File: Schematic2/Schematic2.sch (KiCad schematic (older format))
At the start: 52 parts, among them SW1 Rotary_Encoder_Switch, U1 Kailhlowprofile, U10 Kailhlowprofile, U11 Kailhlowprofile, U12 Kailhlowprofile, U13 Kailhlowprofile, U14 Kailhlowprofile, U15 Kailhlowprofile, U16 Kailhlowprofile, U17 Kailhlowprofile, U18 Kailhlowprofile, U19 Kailhlowprofile, U2 Kailhlowprofile, U20 Kailhlowprofile, U3 Kailhlowprofile, U4 Kailhlowprofile, U5 Kailhlowprofile, U6 Kailhlowprofile, U7 Kailhlowprofile, U8 Kailhlowprofile, U9 Kailhlowprofile

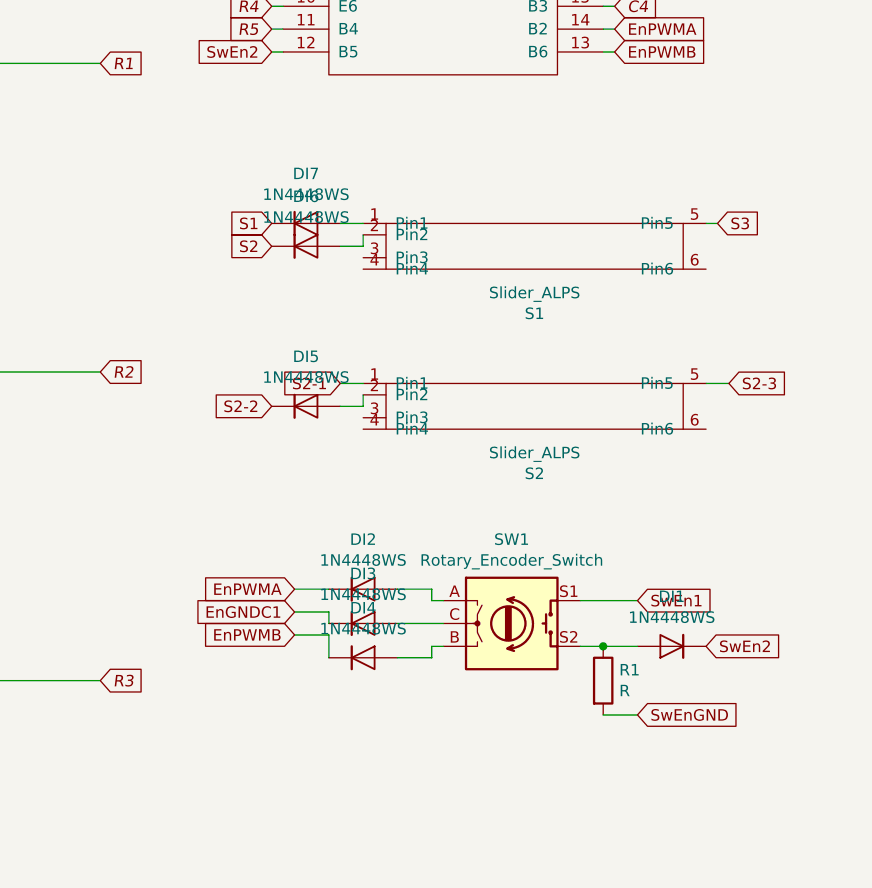
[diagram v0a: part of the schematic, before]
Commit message: The final countdown
The diamond deluxe of FINAL
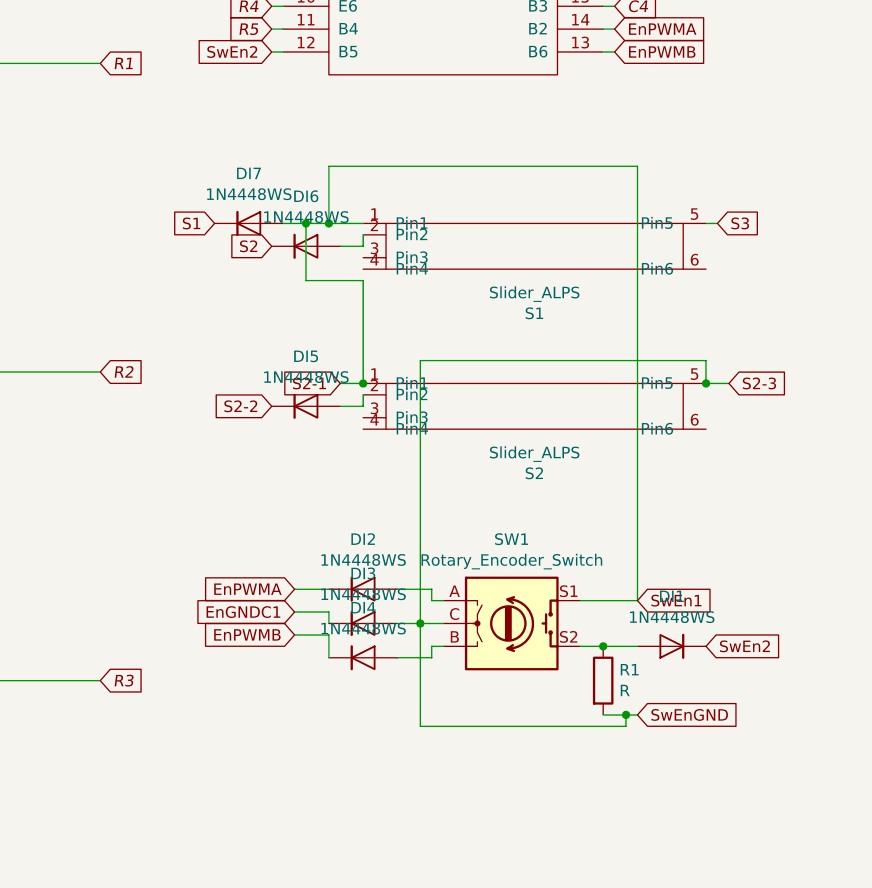
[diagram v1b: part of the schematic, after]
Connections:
- net EnGNDC1: now also DI3.2 (A), SW1.C
- net S1: now also DI7.2 (A), S1.1 (Pin1)
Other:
- moved on the sheet: DI7
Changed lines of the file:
@@
 S3
-Wire Wire Line
-	8850 2650 8950 2650
 Wire Wire Line
 	8850 2750 8950 2750
@@
 Text GLabel 8550 2750 0    50   Input ~ 0
 S2
-Text GLabel 8550 2650 0    50   Input ~ 0
+Text GLabel 8300 2650 0    50   Input ~ 0
 S1
 Text GLabel 10200 1200 2    50   Input ~ 0
@@
 	10000 4500 10150 4500
 Wire Wire Line
-	10000 4800 10150 4800
+	10000 4800 10100 4800
 Text GLabel 10800 900  2    50   Input ~ 0
 SwEnGND
@@
 Wire Wire Line
 	10000 950  10000 900
-Text GLabel 10800 700  2    50   Input ~ 0
-EnGNDC1
 Text GLabel 8650 4350 0    50   Input ~ 0
 EnGNDC1
@@
 L Diode:1N4448WS DI7
 U 1 1 5CAA900B
-P 8700 2650
-F 0 "DI7" H 8700 2867 50  0000 C CNN
-F 1 "1N4448WS" H 8700 2776 50  0000 C CNN
-F 2 "Diode_SMD:D_1206_3216Metric_Pad1.42x1.75mm_HandSolder" H 8700 2475 50  0001 C CNN
-F 3 "https://www.vishay.com/docs/81387/1n4448ws.pdf" H 8700 2650 50  0001 C CNN
-	1    8700 2650
+P 8450 2650
+F 0 "DI7" H 8450 2867 50  0000 C CNN
+F 1 "1N4448WS" H 8450 2776 50  0000 C CNN
+F 2 "Diode_SMD:D_1206_3216Metric_Pad1.42x1.75mm_HandSolder" H 8450 2475 50  0001 C CNN
+F 3 "https://www.vishay.com/docs/81387/1n4448ws.pdf" H 8450 2650 50  0001 C CNN
+	1    8450 2650
 	1    0    0    -1
 $EndComp
@@
 	9250 4250 9250 4300
 Wire Wire Line
-	9100 4400 9300 4400
-Wire Wire Line
 	9100 4550 9250 4550
 Wire Wire Line
@@
 Wire Wire Line
 	10750 950  10000 950
+Text GLabel 10800 700  2    50   Input ~ 0
+EnGNDC1
+Wire Wire Line
+	10100 4850 10100 4800
+Connection ~ 10100 4800
+Wire Wire Line
+	10100 4800 10150 4800
+Wire Wire Line
+	10100 4850 9200 4850
+Wire Wire Line
+	9200 4850 9200 4400
+Wire Wire Line
+	9100 4400 9200 4400
+Wire Wire Line
+	9200 4400 9300 4400
+Connection ~ 9200 4400
+Wire Wire Line
+	10450 3350 10450 3250
+Wire Wire Line
+	10450 3250 9200 3250
+Wire Wire Line
+	9200 3250 9200 4400
+Connection ~ 10450 3350
+Wire Wire Line
+	8600 2650 8700 2650
+Wire Wire Line
+	10150 4300 10150 2400
+Wire Wire Line
+	10150 2400 8800 2400
+Wire Wire Line
+	8800 2400 8800 2650
+Connection ~ 8800 2650
+Wire Wire Line
+	8800 2650 8950 2650
+Wire Wire Line
+	8950 3350 8950 2900
+Wire Wire Line
+	8950 2900 8700 2900
+Wire Wire Line
+	8700 2900 8700 2650
+Connection ~ 8950 3350
+Connection ~ 8700 2650
+Wire Wire Line
+	8700 2650 8800 2650
 $EndSCHEMATC
